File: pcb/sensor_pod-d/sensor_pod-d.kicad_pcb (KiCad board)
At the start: 2 copper layers, 20.2 x 20.2 mm, 8 parts, among them J2 Conn_01x04_Socket, Q2 Q_Photo_NPN

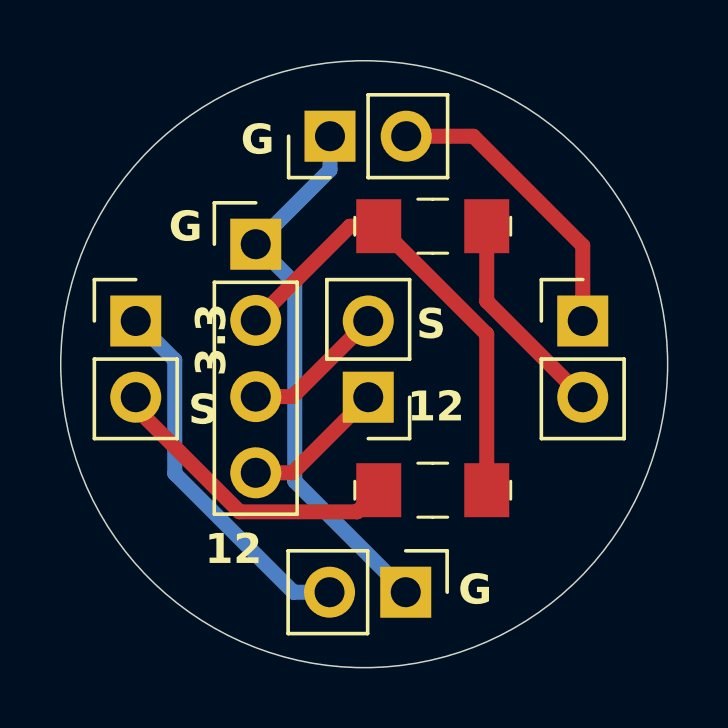
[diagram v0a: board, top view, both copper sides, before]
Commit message: PCB fixes and adjustments
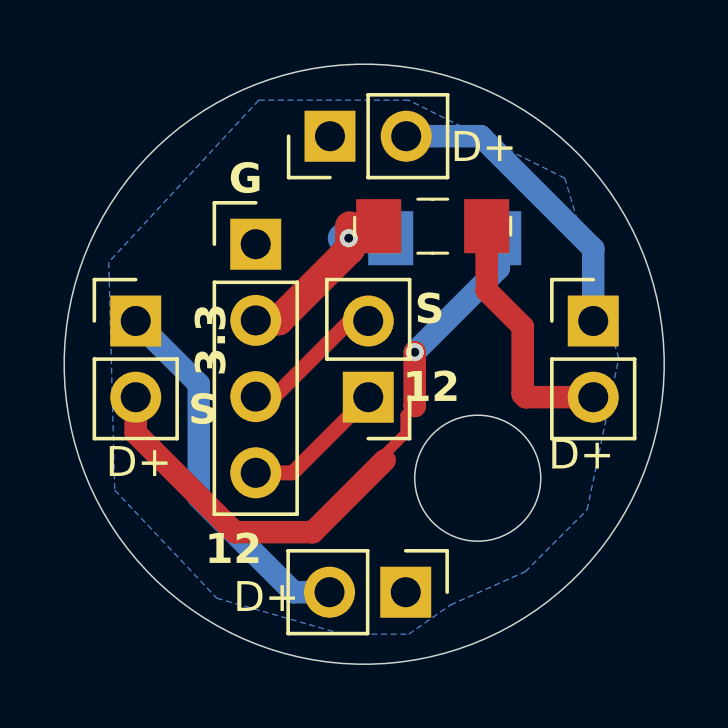
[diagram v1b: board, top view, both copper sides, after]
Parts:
- R4: moved to B.Cu
- moved R4 8.41 mm to (167.8, 92.2), turned to 0 degrees
- moved D1 0.35 mm to (172.8, 95.0)
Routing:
- net GND: track 18.3 -> 0.00 mm
- net Net-(D3-A): track 10.2 -> 21.2 mm, vias 0 -> 1
- net /3.3: track 15.7 -> 7.61 mm, vias 0 -> 1
- net Net-(D1-A): track 7.03 -> 8.66 mm
- added copper zone on B.Cu, net GND
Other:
- board size 20.2 x 20.2 mm -> 20 x 20 mm
- rule pad_to_mask_clearance: 0 -> 0.0508
- board text added: "D+"
